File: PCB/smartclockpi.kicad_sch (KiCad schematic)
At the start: 22 parts, among them J1 Raspberry_Pi, J2 DS3231 RTC module, J3 ILI9488 SPI TFT touchscreen, J4 PCM5102A DAC (with headphone 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, J5 USB_B_Micro, J6 USB_A, J7 microUSB IN, J8 USB-A OUT, J9 PWR IN, U2 MCP3008, U3 DHT22

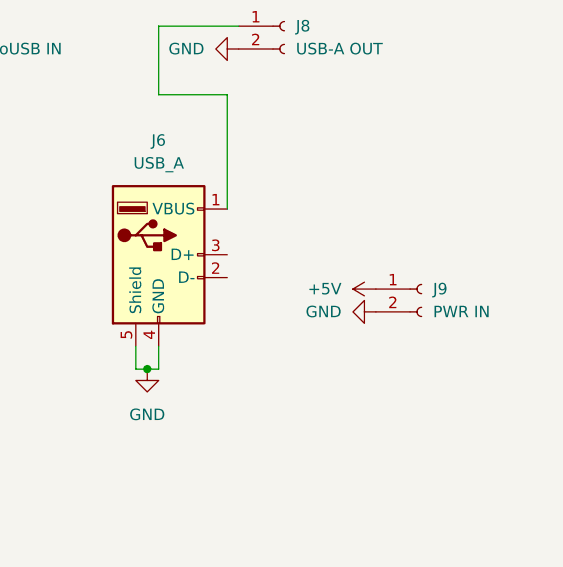
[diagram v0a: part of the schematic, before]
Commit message: update PCB
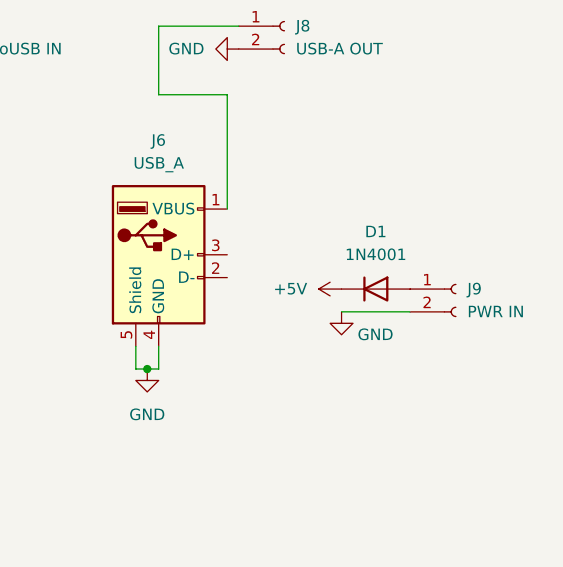
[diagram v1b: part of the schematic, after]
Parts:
- added D1: 1N4001, Diode_THT:D_DO-41_SOD81_P10.16mm_Horizontal, symbol Diode:1N4001
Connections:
- net +5V: now also D1.1 (K); no longer J9.1 (Pin_1)
- new net: D1.2 (A), J9.1 (Pin_1)
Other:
- moved on the sheet: J9
